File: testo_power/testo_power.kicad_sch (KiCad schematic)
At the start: 1 part, among them J1 USB_C_Receptacle_PowerOnly_6P

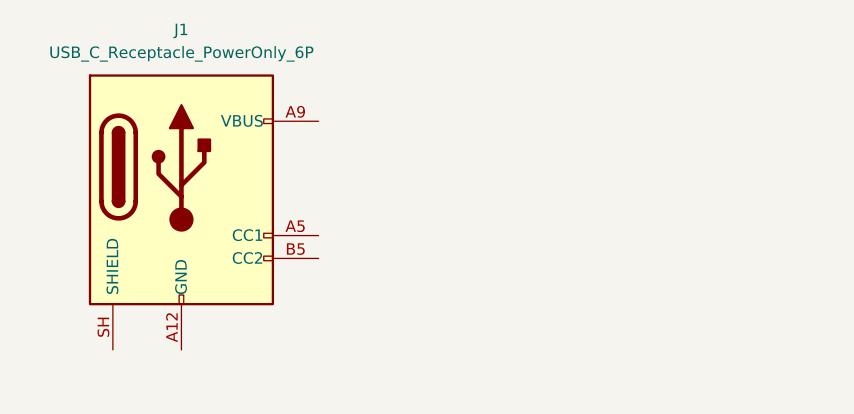
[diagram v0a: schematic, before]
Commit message: added random component
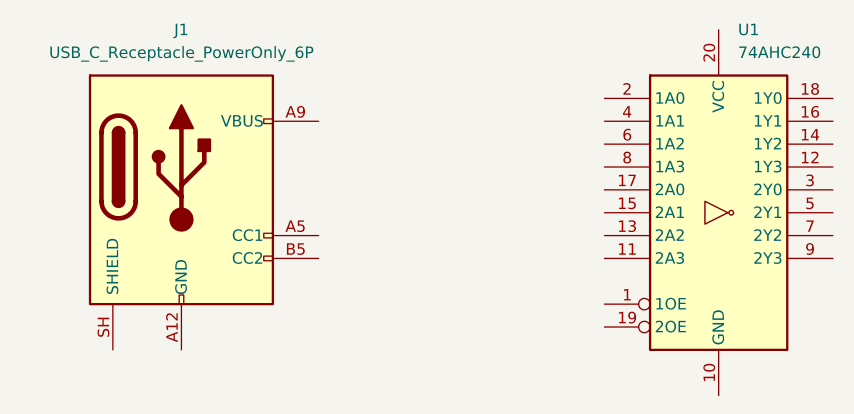
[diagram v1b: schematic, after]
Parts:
- added U1: 74AHC240, symbol 74xx:74AHC240
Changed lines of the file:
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@@
 	(paper "A4")
+	(symbol
+		(lib_id "74xx:74AHC240")
+		(at 134.62 73.66 0)
+		(unit 1)
+		(body_style 1)
+		(exclude_from_sim no)
+		(in_bom yes)
+		(on_board yes)
+		(in_pos_files yes)
+		(dnp no)
+		(fields_autoplaced yes)
+		(property "Reference" "U1"
+			(at 136.7633 53.34 0)
+			(show_name no)
+			(do_not_autoplace no)
+			(effects
+				(font
+					(size 1.27 1.27)
+				)
+				(justify left)
+			)
+		)
+		(property "Value" "74AHC240"
+			(at 136.7633 55.88 0)
+			(show_name no)
+			(do_not_autoplace no)
+			(effects
+				(font
+					(size 1.27 1.27)
+				)
+				(justify left)
+			)
+		)
+		(property "Footprint" ""
+			(at 134.62 73.66 0)
+			(hide yes)
+			(show_name no)
+			(do_not_autoplace no)
+			(effects
+				(font
+					(size 1.27 1.27)
+				)
+			)
+		)
+		(property "Datasheet" "https://www.ti.com/lit/ds/symlink/sn54ahc240.pdf"
+			(at 134.62 73.66 0)
+			(hide yes)
+			(show_name no)
+			(do_not_autoplace no)
+			(effects
+				(font
+					(size 1.27 1.27)
+				)
+			)
+		)
+		(property "Description" "8-bit Buffer/Line Driver 3-state Inverting"
+			(at 134.62 73.66 0)
+			(hide yes)
+			(show_name no)
+			(do_not_autoplace no)
+			(effects
+				(font
+					(size 1.27 1.27)
+				)
+			)
+		)
+		(pin "14"
+		)
+		(pin "15"
+		)
+		(pin "10"
+		)
+		(pin "13"
+		)
+		(pin "8"
+		)
+		(pin "12"
+		)
+		(pin "11"
+		)
+		(pin "19"
+		)
+		(pin "7"
+		)
+		(pin "4"
+		)
+		(pin "6"
+		)
+		(pin "3"
+		)
+		(pin "5"
+		)
+		(pin "2"
+		)
+		(pin "1"
+		)
+		(pin "20"
+		)
+		(pin "17"
+		)
+		(pin "18"
+		)
+		(pin "16"
+		)
+		(pin "9"
+		)
+		(instances
+			(project "testo_power"
+				(path "/7d8517b7-4e53-4e94-8436-66e52bec9654"
+					(reference "U1")
+					(unit 1)
+				)
+			)
+		)
+	)
 	(symbol
 		(lib_id "Connector:USB_C_Receptacle_PowerOnly_6P")
